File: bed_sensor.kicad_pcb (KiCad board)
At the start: 2 copper layers, 41 x 36 mm, 32 parts, among them J1 Conn_01x02, J2 Conn_01x06, J3 ISP, J4 Conn_01x02, J5 DM3AT-SF-PEJM5, Q1 2N2219, SW1 SW_SPST, U1 MIC5205-3.3, U2 MPU-9250, U3 ATMEGA328-AU, U5 CFAH0802D-YYH-JP, Y1 Crystal_GND2

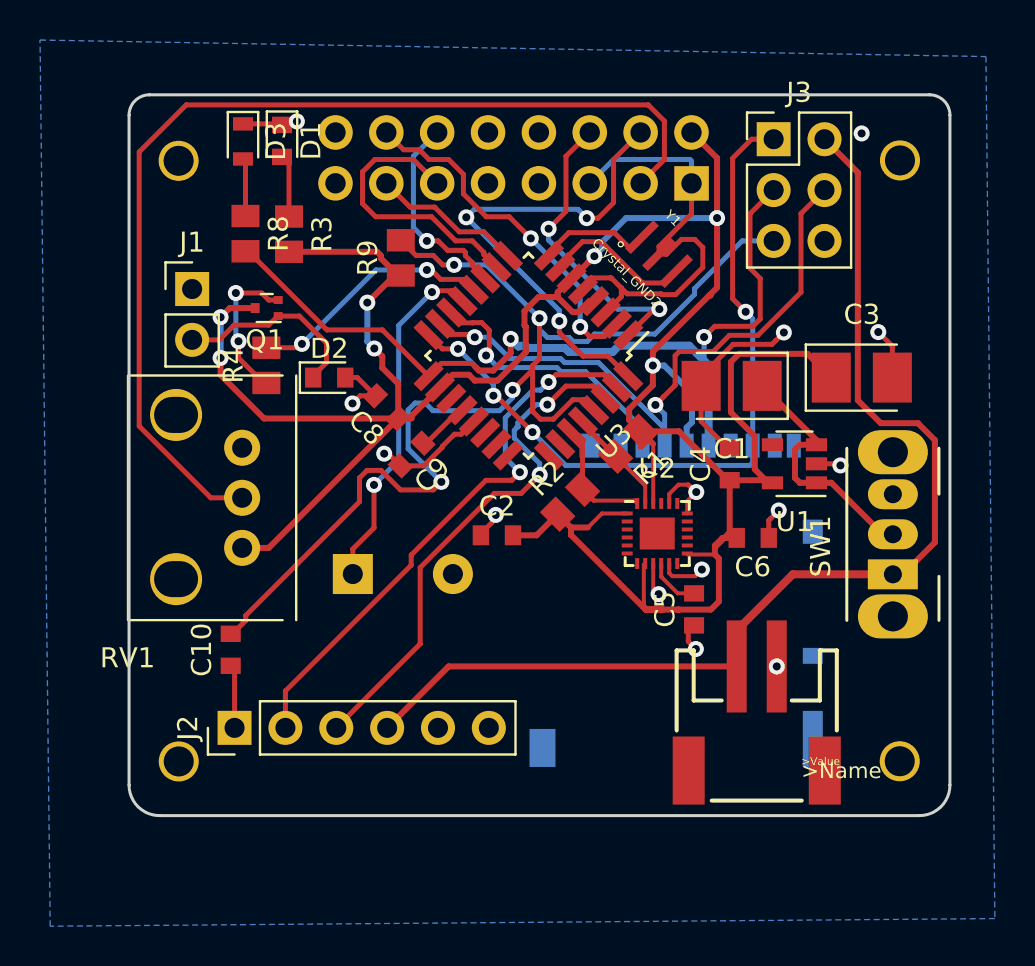
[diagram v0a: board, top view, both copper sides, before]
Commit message: cleaned up board
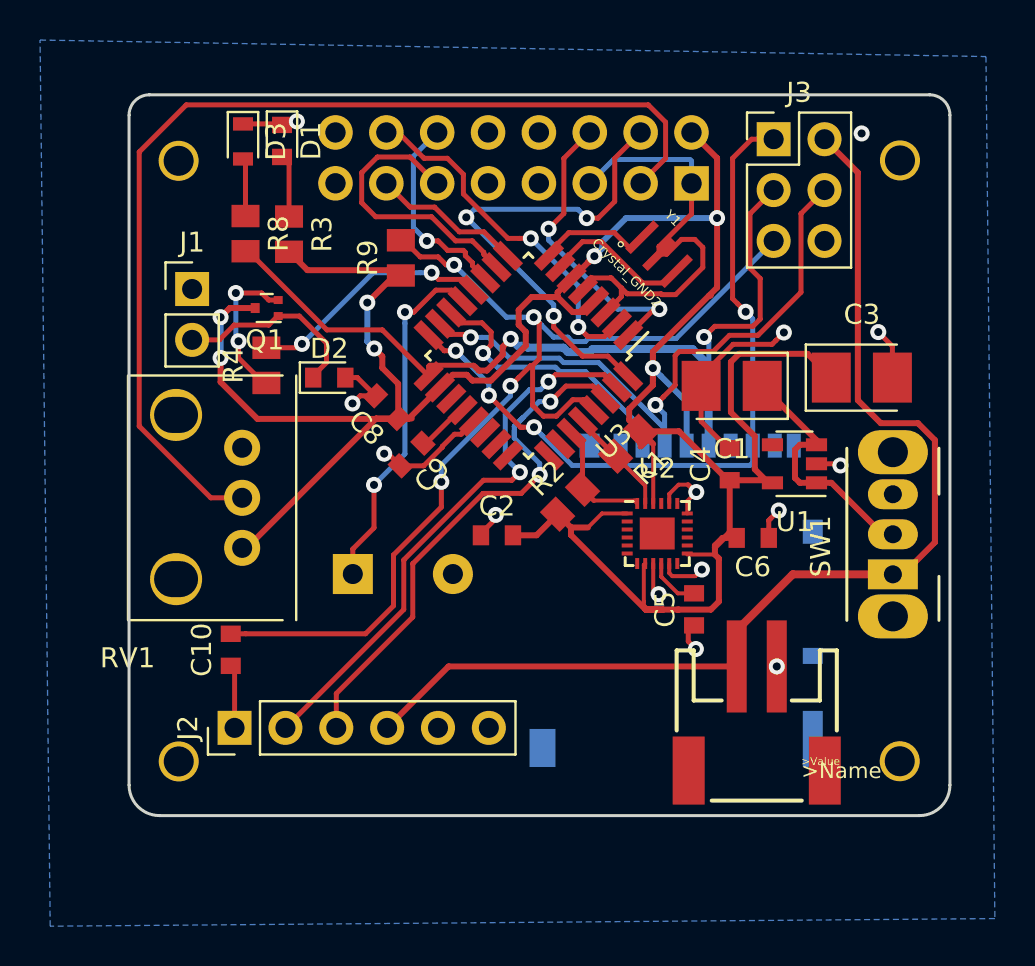
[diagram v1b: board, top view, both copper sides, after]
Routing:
- net /Ardunio/RESET: track 59.4 -> 55.0 mm
- net /Ardunio/RX1: track 26.3 -> 27.9 mm
